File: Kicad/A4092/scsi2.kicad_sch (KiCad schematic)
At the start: 28 parts, among them J3 TO-LED, J4 TO-MB, J8 TO-A3000-LED, J9 TO-A3000-MB, U10 NCR53c710 SCSI Host Controller, Y1 Abracon ACO-50MHz

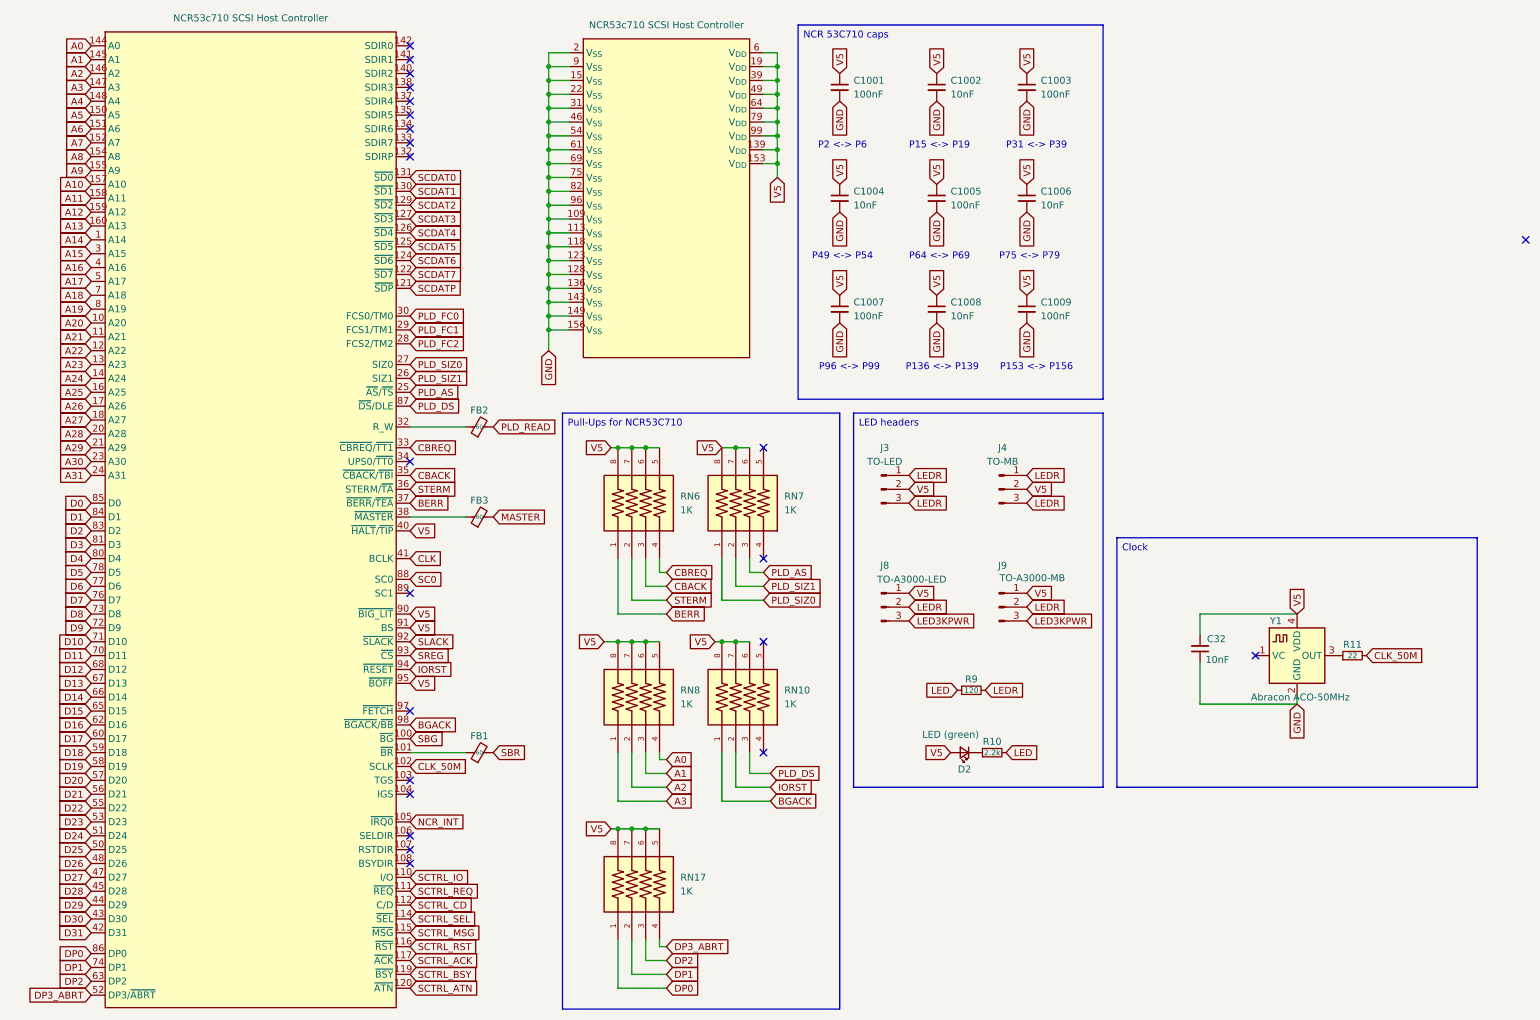
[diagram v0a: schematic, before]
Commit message: First version of A4770 cheetah
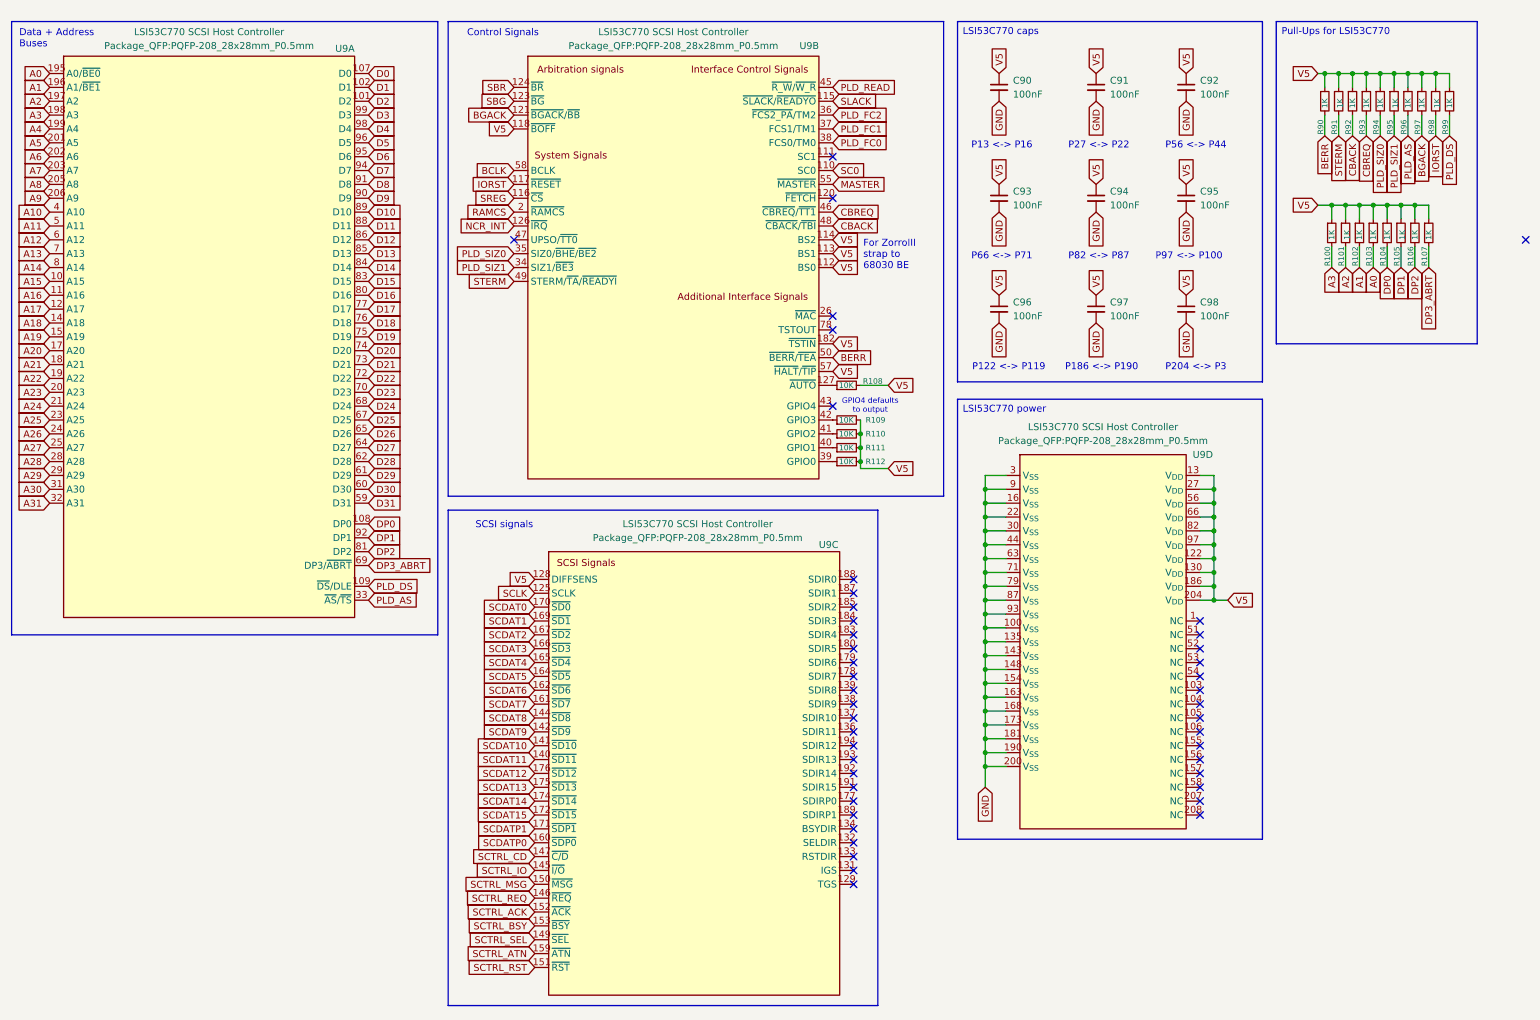
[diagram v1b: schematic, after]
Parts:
- removed C32: 10nF, Capacitor_SMD:C_0603_1608Metric_Pad1.08x0.95mm_HandSolder, symbol Device:C_Small
- removed D2: LED (green), LED_SMD:LED_0805_2012Metric, symbol Device:LED_Small
- removed FB1, FB2, FB3: 60, Capacitor_SMD:C_0603_1608Metric_Pad1.08x0.95mm_HandSolder, symbol Device:FerriteBead_Small
- removed J3: TO-LED, Connector_PinHeader_2.54mm:PinHeader_1x03_P2.54mm_Vertical, symbol Connector:Conn_01x03_Pin
- removed J4: TO-MB, Connector_PinHeader_2.54mm:PinHeader_1x03_P2.54mm_Vertical, symbol Connector:Conn_01x03_Pin
- removed J8: TO-A3000-LED, Connector_PinHeader_2.54mm:PinHeader_1x03_P2.54mm_Vertical, symbol Connector:Conn_01x03_Pin
- removed J9: TO-A3000-MB, Connector_PinHeader_2.54mm:PinHeader_1x03_P2.54mm_Vertical, symbol Connector:Conn_01x03_Pin
- removed R10: 2.2k, Resistor_SMD:R_0603_1608Metric, symbol Device:R_Small
- removed R11: 22, Resistor_SMD:R_0603_1608Metric, symbol Device:R_Small
- removed R9: 120, Resistor_SMD:R_0603_1608Metric, symbol Device:R_Small
- removed RN10, RN17, RN6, RN7, RN8: 1K, CAY16_102J4LF:BO_CAY16, symbol YC324-FK-071KL:YC324-FK-071KL
- removed U10: NCR53c710 SCSI Host Controller, Package_QFP:PQFP-160_28x28mm_P0.65mm, symbol NCRSCSI:NCR53c710
- removed Y1: Abracon ACO-50MHz, Oscillator:Oscillator_SMD_Fox_FT5H_5.0x3.2mm, symbol Oscillator:FT5HV
- added R100, R101, R102, R103, R104, R105, R106, R107, R90, R91, R92, R93, R94, R95, R96, R97, R98, R99: 1K, Resistor_SMD:R_0603_1608Metric_Pad0.98x0.95mm_HandSolder, symbol Device:R_Small
- added R108, R109, R110, R111, R112: 10K, Resistor_SMD:R_0603_1608Metric_Pad0.98x0.95mm_HandSolder, symbol Device:R_Small
- added U9: LSI53C770 SCSI Host Controller, Package_QFP:PQFP-208_28x28mm_P0.5mm, symbol NCRSCSI:LSI53C770
- C91: renamed from C1002; value 10nF -> 100nF
- C93: renamed from C1004; value 10nF -> 100nF
- C95: renamed from C1006; value 10nF -> 100nF
- C97: renamed from C1008; value 10nF -> 100nF
- renumbered C1001 to C90, C1003 to C92, C1005 to C94, C1007 to C96, C1009 to C98
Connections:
- net A0: now also R103.2, U9.195 (A0/~{BE0})
- net A1: now also R102.2, U9.196 (A1/~{BE1})
- net A10: now also U9.4 (A10)
- net A11: now also U9.5 (A11)
- net A12: now also U9.6 (A12)
- net A13: now also U9.7 (A13)
- net A14: now also U9.8 (A14)
- net A15: now also U9.10 (A15)
- net A16: now also U9.11 (A16)
- net A17: now also U9.12 (A17)
- net A18: now also U9.14 (A18)
- net A19: now also U9.15 (A19)
- net A2: now also R101.2, U9.197 (A2)
- net A20: now also U9.17 (A20)
- net A21: now also U9.18 (A21)
- net A22: now also U9.19 (A22)
- net A23: now also U9.20 (A23)
- net A24: now also U9.21 (A24)
- net A25: now also U9.23 (A25)
- net A26: now also U9.24 (A26)
- net A27: now also U9.25 (A27)
- net A28: now also U9.28 (A28)
- net A29: now also U9.29 (A29)
- net A3: now also R100.2, U9.198 (A3)
- net A30: now also U9.31 (A30)
- net A31: now also U9.32 (A31)
- net A4: now also U9.199 (A4)
- net A5: now also U9.201 (A5)
- net A6: now also U9.202 (A6)
- net A7: now also U9.203 (A7)
- net A8: now also U9.205 (A8)
- net A9: now also U9.206 (A9)
- net BERR: now also R90.2, U9.50 (~{BERR}/~{TEA})
- net BGACK: now also R97.2, U9.121 (~{BGACK}/~{BB})
- net CBACK: now also R92.2, U9.48 (~{CBACK}/~{TBI})
- net CBREQ: now also R93.2, U9.46 (~{CBREQ}/~{TT1})
- net D0: now also U9.107 (D0)
- net D1: now also U9.102 (D1)
- net D10: now also U9.89 (D10)
- net D11: now also U9.88 (D11)
- net D12: now also U9.86 (D12)
- net D13: now also U9.85 (D13)
- net D14: now also U9.84 (D14)
- net D15: now also U9.83 (D15)
- net D16: now also U9.80 (D16)
- net D17: now also U9.77 (D17)
- net D18: now also U9.76 (D18)
- net D19: now also U9.75 (D19)
- net D2: now also U9.101 (D2)
- net D20: now also U9.74 (D20)
- net D21: now also U9.73 (D21)
- net D22: now also U9.72 (D22)
- net D23: now also U9.70 (D23)
- net D24: now also U9.68 (D24)
- net D25: now also U9.67 (D25)
- net D26: now also U9.65 (D26)
- net D27: now also U9.64 (D27)
- net D28: now also U9.62 (D28)
- net D29: now also U9.61 (D29)
- net D3: now also U9.99 (D3)
- net D30: now also U9.60 (D30)
- net D31: now also U9.59 (D31)
- net D4: now also U9.98 (D4)
- net D5: now also U9.96 (D5)
- net D6: now also U9.95 (D6)
- net D7: now also U9.94 (D7)
- net D8: now also U9.91 (D8)
- net D9: now also U9.90 (D9)
- net DP0: now also R104.2, U9.108 (DP0)
- net DP1: now also R105.2, U9.92 (DP1)
- net DP2: now also R106.2, U9.81 (DP2)
- net DP3_ABRT: now also R107.2, U9.69 (DP3/~{ABRT})
- net GND: now also U9.100 (V_{SS}), U9.135 (V_{SS}), U9.143 (V_{SS}), U9.148 (V_{SS}), U9.154 (V_{SS}), U9.16 (V_{SS}), U9.163 (V_{SS}), U9.168 (V_{SS}), U9.173 (V_{SS}), U9.181 (V_{SS}), U9.190 (V_{SS}), U9.200 (V_{SS}), U9.22 (V_{SS}), U9.3 (V_{SS}), U9.30 (V_{SS}), U9.44 (V_{SS}), U9.63 (V_{SS}), U9.71 (V_{SS}), U9.79 (V_{SS}), U9.87 (V_{SS}), U9.9 (V_{SS}), U9.93 (V_{SS})
- net IORST: now also R98.2, U9.117 (~{RESET})
- net MASTER: now also U9.55 (~{MASTER})
- net NCR_INT: now also U9.126 (~{IRQ})
- net PLD_AS: now also R96.2, U9.33 (~{AS}/~{TS})
- net PLD_DS: now also R99.2, U9.109 (~{DS}/DLE)
- net PLD_FC0: now also U9.38 (FCS0/TM0)
- net PLD_FC1: now also U9.37 (FCS1/TM1)
- net PLD_FC2: now also U9.36 (~{FCS2_PA}/TM2)
- net PLD_READ: now also U9.45 (~{R_W}/~{W_R})
- net PLD_SIZ0: now also R94.2, U9.35 (SIZ0/~{BHE}/~{BE2})
- net PLD_SIZ1: now also R95.2, U9.34 (SIZ1/~{BE3})
- net SBG: now also U9.123 (~{BG})
- net SBR: now also U9.124 (~{BR})
- net SC0: now also U9.110 (SC0)
- net SCDAT0: now also U9.170 (~{SD0})
- net SCDAT1: now also U9.169 (~{SD1})
- net SCDAT2: now also U9.167 (~{SD2})
- net SCDAT3: now also U9.166 (~{SD3})
- net SCDAT4: now also U9.165 (~{SD4})
- net SCDAT5: now also U9.164 (~{SD5})
- net SCDAT6: now also U9.162 (~{SD6})
- net SCDAT7: now also U9.161 (~{SD7})
- net SCTRL_ACK: now also U9.152 (~{ACK})
- net SCTRL_ATN: now also U9.159 (~{ATN})
- net SCTRL_BSY: now also U9.153 (~{BSY})
- net SCTRL_CD: now also U9.147 (~{C/D})
- net SCTRL_IO: now also U9.145 (~{I/O})
- net SCTRL_MSG: now also U9.150 (~{MSG})
- net SCTRL_REQ: now also U9.146 (~{REQ})
- net SCTRL_RST: now also U9.151 (~{RST})
- net SCTRL_SEL: now also U9.149 (~{SEL})
- net SLACK: now also U9.115 (~{SLACK}/~{READYO})
- net SREG: now also U9.116 (~{CS})
- net STERM: now also R91.2, U9.49 (STERM/~{TA}/~{READYI})
- net V5: now also R100.1, R101.1, R102.1, R103.1, R104.1, R105.1, R106.1, R107.1, R108.2, R109.2, R110.2, R111.2, R112.2, R90.1, R91.1, R92.1, R93.1, R94.1, R95.1, R96.1, R97.1, R98.1, R99.1, U9.112 (BS0), U9.113 (BS1), U9.114 (BS2), U9.118 (~{BOFF}), U9.122 (V_{DD}), U9.128 (DIFFSENS), U9.13 (V_{DD}), U9.130 (V_{DD}), U9.182 (~{TSTIN}), U9.186 (V_{DD}), U9.204 (V_{DD}), U9.27 (V_{DD}), U9.56 (V_{DD}), U9.57 (~{HALT}/~{TIP}), U9.66 (V_{DD}), U9.82 (V_{DD}), U9.97 (V_{DD})
- new net: R108.1, U9.127 (~{AUTO})
- new net: R112.1, U9.39 (GPIO0)
- new net: R111.1, U9.40 (GPIO1)
- new net: R110.1, U9.41 (GPIO2)
- new net: R109.1, U9.42 (GPIO3)
- new net BCLK: U9.58 (BCLK)
- new net RAMCS: U9.2 (~{RAMCS})
- new net SCDAT10: U9.141 (~{SD10})
- new net SCDAT11: U9.140 (~{SD11})
- new net SCDAT12: U9.176 (~{SD12})
- new net SCDAT13: U9.175 (~{SD13})
- new net SCDAT14: U9.174 (~{SD14})
- new net SCDAT15: U9.172 (~{SD15})
- new net SCDAT8: U9.144 (~{SD8})
- new net SCDAT9: U9.142 (~{SD9})
- new net SCDATP0: U9.160 (~{SDP0})
- new net SCDATP1: U9.171 (~{SDP1})
- new net SCLK: U9.125 (SCLK)
- no-connect marks 23 -> 45
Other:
- note added: "Control Signals"
- note added: "Data + Address Buses"
- note added: "For ZorroIII strap to 68030 BE"
- note added: "GPIO4 defaults to output"
- note added: "P122 <-> P119"
- note added: "P13 <-> P16"
- note added: "P186 <-> P190"
- note added: "P204 <-> P3"
- note added: "P27 <-> P22"
- note added: "P56 <-> P44"
- note added: "P66 <-> P71"
- note added: "P82 <-> P87"
- note added: "P97 <-> P100"
- note added: "SCSI signals"
- note removed: "P136 <-> P139"
- note removed: "P15 <-> P19"
- note removed: "P153 <-> P156"
- note removed: "P2 <-> P6"
- note removed: "P31 <-> P39"
- note removed: "P49 <-> P54"
- note removed: "P64 <-> P69"
- note removed: "P75 <-> P79"
- note removed: "P96 <-> P99"
- moved on the sheet: C90, C91, C92, C93, C94, C95, C96, C97, C98
